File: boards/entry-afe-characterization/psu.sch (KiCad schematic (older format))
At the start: 45 parts, among them J10 CONN_3_PWROUT, U10 LT3042, U11 LT3042, U12 MCP1501T-25E/RW, U8 TPS54227-DRC, U9 LT3042

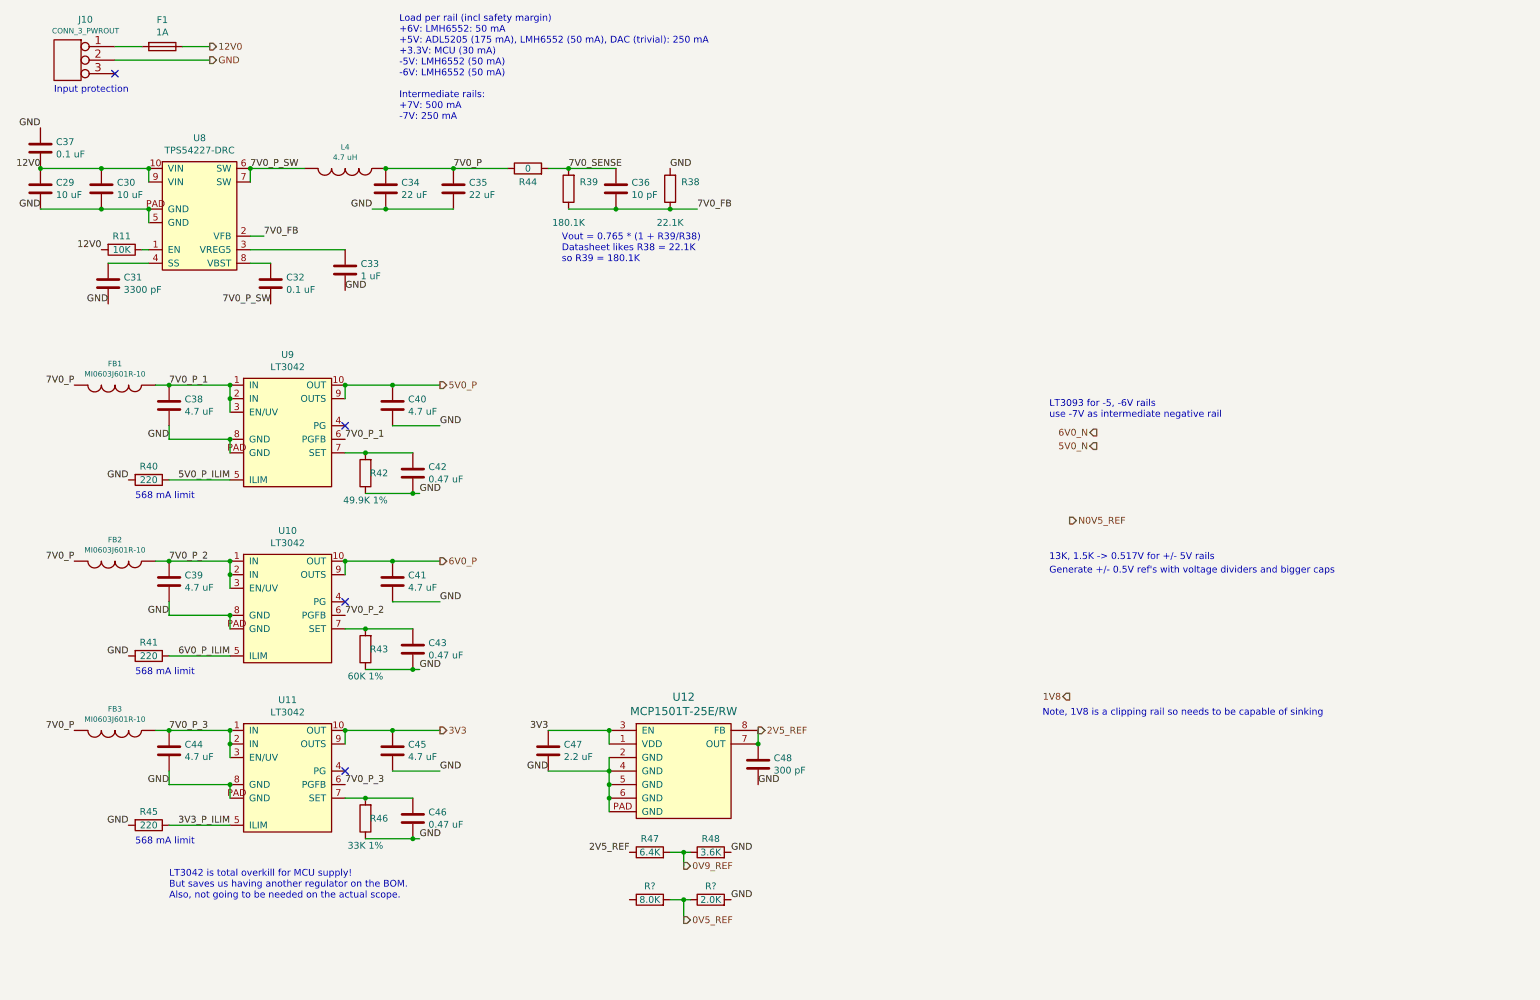
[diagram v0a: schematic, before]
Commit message: Final iteration of entry-afe-characterization, ready for schematic review
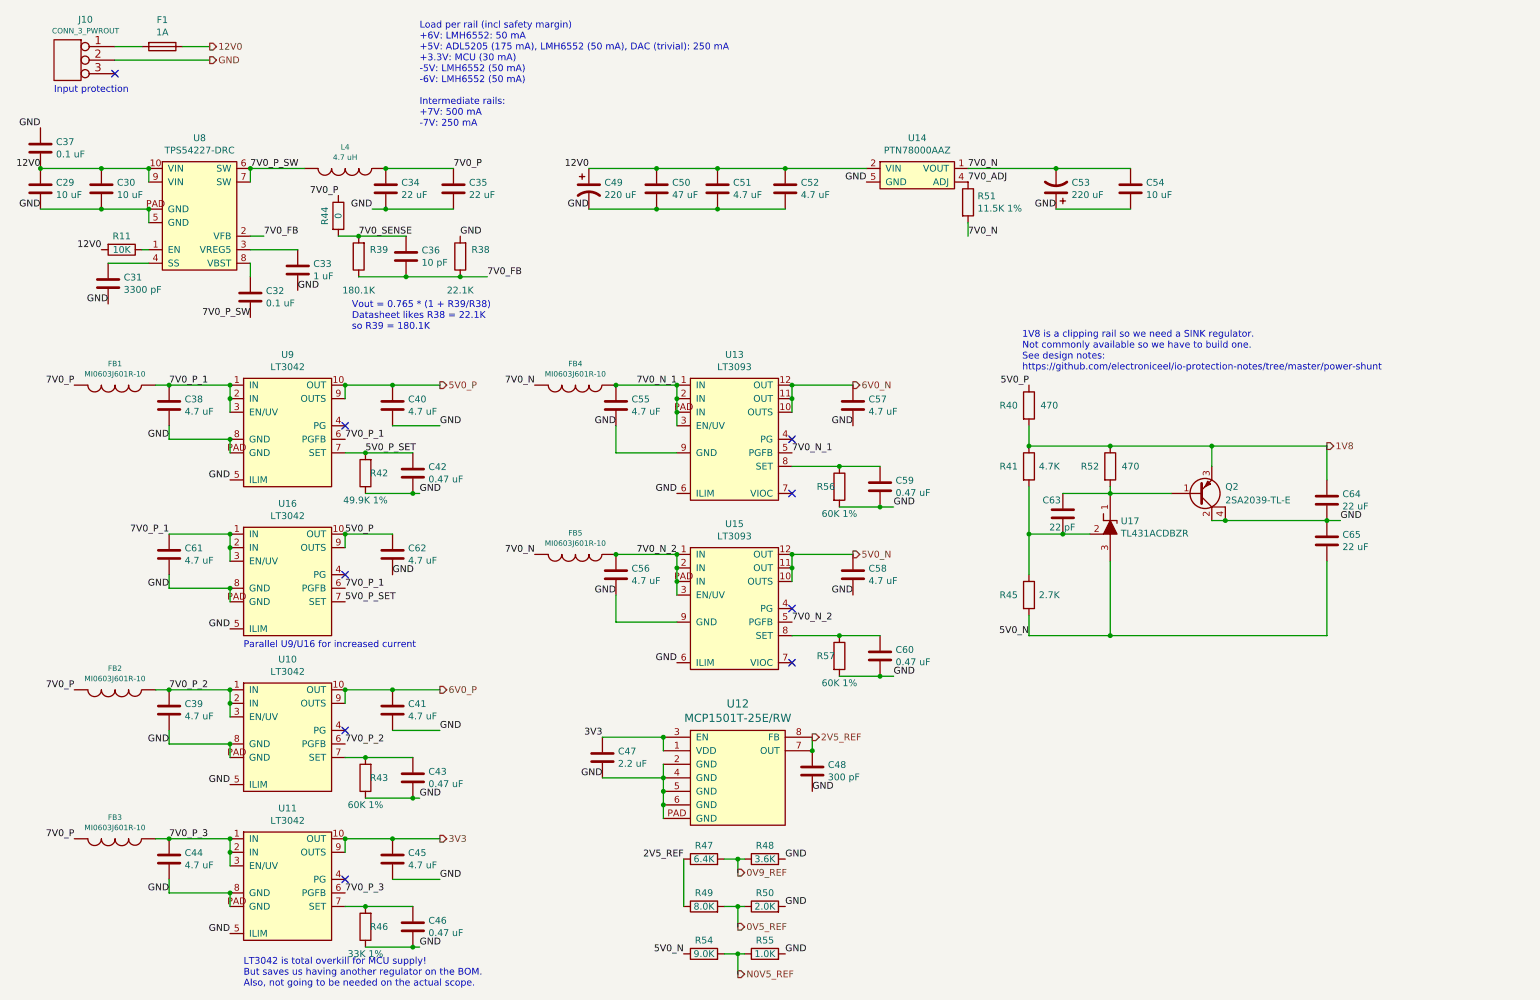
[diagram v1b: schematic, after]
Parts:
- added C49, C53: 220 uF, symbol device:CP1
- added C50: 47 uF, symbol device:C
- added C51, C52, C55, C56, C57, C58, C61, C62: 4.7 uF, symbol device:C
- added C54: 10 uF, symbol device:C
- added C59, C60: 0.47 uF, symbol device:C
- added C63: 22 pF, symbol device:C
- added C64, C65: 22 uF, symbol device:C
- added FB4, FB5: MI0603J601R-10, symbol passive-azonenberg:INDUCTOR_PWROUT
- added Q2: 2SA2039-TL-E, symbol device:Q_PNP_BCEC
- added R51: 11.5K 1%, symbol device:R
- added R52: 470, symbol device:R
- added R54: 9.0K, symbol device:R
- added R55: 1.0K, symbol device:R
- added R56, R57: 60K 1%, symbol device:R
- added U13, U15: LT3093, symbol power-azonenberg:LT3093
- added U14: PTN78000AAZ, symbol power-azonenberg:PTN78000AAZ
- added U16: LT3042, symbol power-azonenberg:LT3042
- added U17: TL431ACDBZR, symbol analog-azonenberg:TL431A_SOT23_TI_DBZ
- R40: value 220 -> 470
- R41: value 220 -> 4.7K
- R45: value 220 -> 2.7K
- gave numbers to parts that had none: 2
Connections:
- net 12V0: now also C49.1, C50.1, C51.1, C52.1, U14.2 (VIN)
- net 1V8: now also R40.2, R41.1, C64.1, Q2.3 (E), R52.1
- net 2V5_REF: now also R49.1
- net 5V0_N: now also R45.2, C58.1, C65.2, R54.1, U15.10 (OUTS), U15.11 (OUT), U15.12 (OUT), U17.3
- net 5V0_P: now also R40.1, C62.1, U16.10 (OUT), U16.9 (OUTS)
- net 6V0_N: now also C57.1, U13.10 (OUTS), U13.11 (OUT), U13.12 (OUT)
- net 7V0_P_1: now also C61.1, U16.1 (IN), U16.2 (IN), U16.3 (EN/UV), U16.6 (PGFB)
- net GND: now also U10.5 (ILIM), U11.5 (ILIM), U9.5 (ILIM), C49.2, C50.2, C51.2, C52.2, C53.1, C54.2, C55.2, C56.2, C57.2, C58.2, C59.2, C60.2, C61.2, C62.2, C64.2, C65.1, Q2.2 (C), Q2.4 (C), R55.2, R56.2, R57.2, U13.6 (ILIM), U13.9 (GND), U14.5 (GND), U15.6 (ILIM), U15.9 (GND), U16.5 (ILIM), U16.8 (GND), U16.PAD (GND); no longer R40.2, R41.2, R45.2
- net N0V5_REF: now also R54.2, R55.1
- net 5V0_P_SET: now reaches C42.1, R42.2, U9.7 (SET)
- net 5V0_P_SET: now also U16.7 (SET)
- net 3V3_P_ILIM: no longer names the net of R45.1
- net 3V3_P_ILIM: now also R41.2, C63.2, U17.2; no longer U11.5 (ILIM)
- removed net 5V0_P_ILIM: R40.1, U9.5 (ILIM)
- removed net 6V0_P_ILIM: R41.1, U10.5 (ILIM)
- new net: C59.1, R56.1, U13.8 (SET)
- new net: C60.1, R57.1, U15.8 (SET)
- new net: C63.1, Q2.1 (B), R52.2, U17.1
- new net 7V0_ADJ: R51.1, U14.4 (ADJ)
- new net 7V0_N: C53.2, C54.1, FB4.2, FB5.2, R51.2, U14.1 (VOUT)
- new net 7V0_N_1: C55.1, FB4.1, U13.1 (IN), U13.2 (IN), U13.3 (EN/UV), U13.5 (PGFB), U13.PAD (IN)
- new net 7V0_N_2: C56.1, FB5.1, U15.1 (IN), U15.2 (IN), U15.3 (EN/UV), U15.5 (PGFB), U15.PAD (IN)
- no-connect marks 4 -> 9
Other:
- note added: "1V8 is a clipping rail so we need a SINK regulator.\nNot commonly available so we have to build one.\nSee design notes:\nhttps://github.com/electroniceel/io-protection-notes/tree/master/power-shunt"
- note added: "Parallel U9/U16 for increased current"
- note removed: "13K, 1.5K -> 0.517V for +/- 5V rails"
- note removed: "568 mA limit"
- note removed: "Generate +/- 0.5V ref's with voltage dividers and bigger caps"
- note removed: "LT3093 for -5, -6V rails\nuse -7V as intermediate negative rail"
- note removed: "Note, 1V8 is a clipping rail so needs to be capable of sinking"
- moved on the sheet: C32, C33, C36, C39, C41, C43, C44, C45, C46, C47, C48, FB2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
